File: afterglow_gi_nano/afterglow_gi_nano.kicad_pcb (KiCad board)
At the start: 2 copper layers, 52 parts, among them J1 Conn_02x17_Odd_Even, J2 POWER_CONN, J3 GI_WPC_J120, J4 GI_WPC_J121, J5 GI_CONN_J119, Q1 FQP30N06L, Q2 FQP30N06L, Q3 FQP30N06L, Q4 FQP30N06L, Q5 FQP30N06L, U1 74LS374, U2 L7805

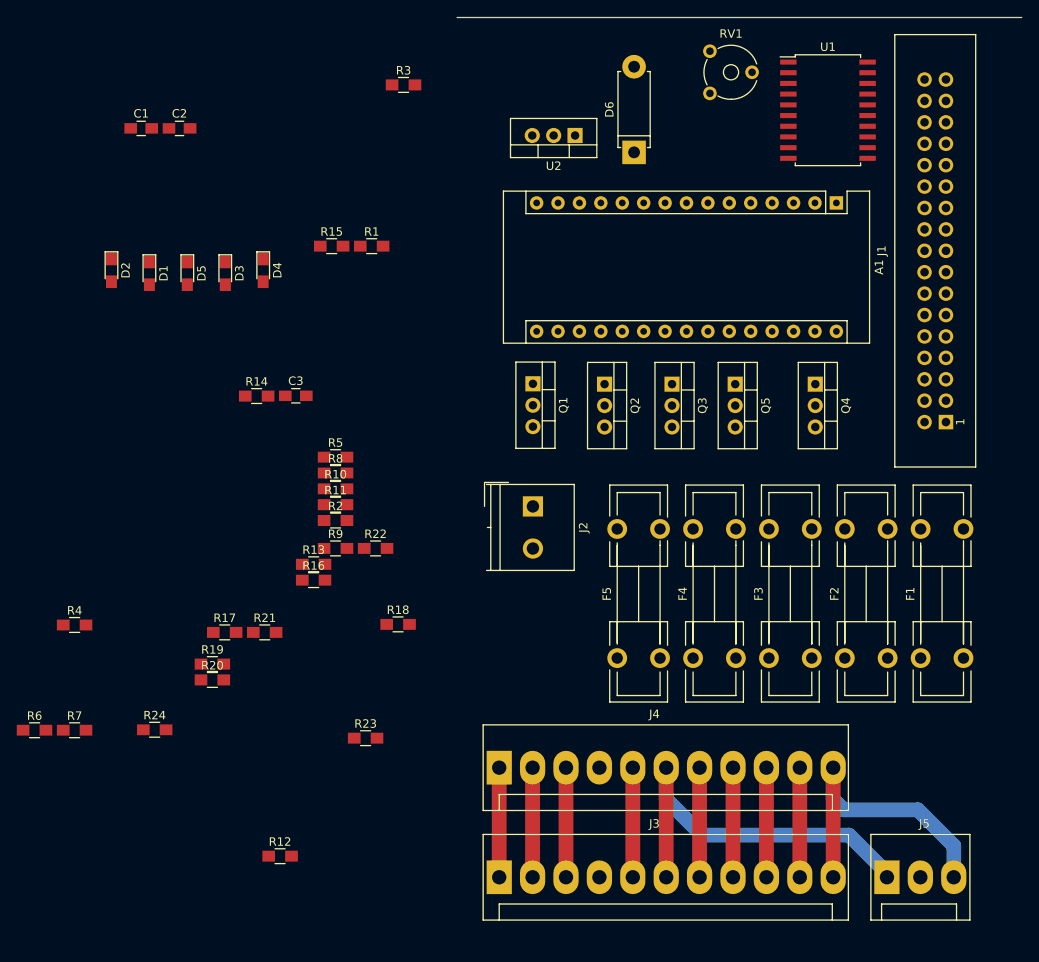
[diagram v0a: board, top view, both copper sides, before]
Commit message: Some PCB progress
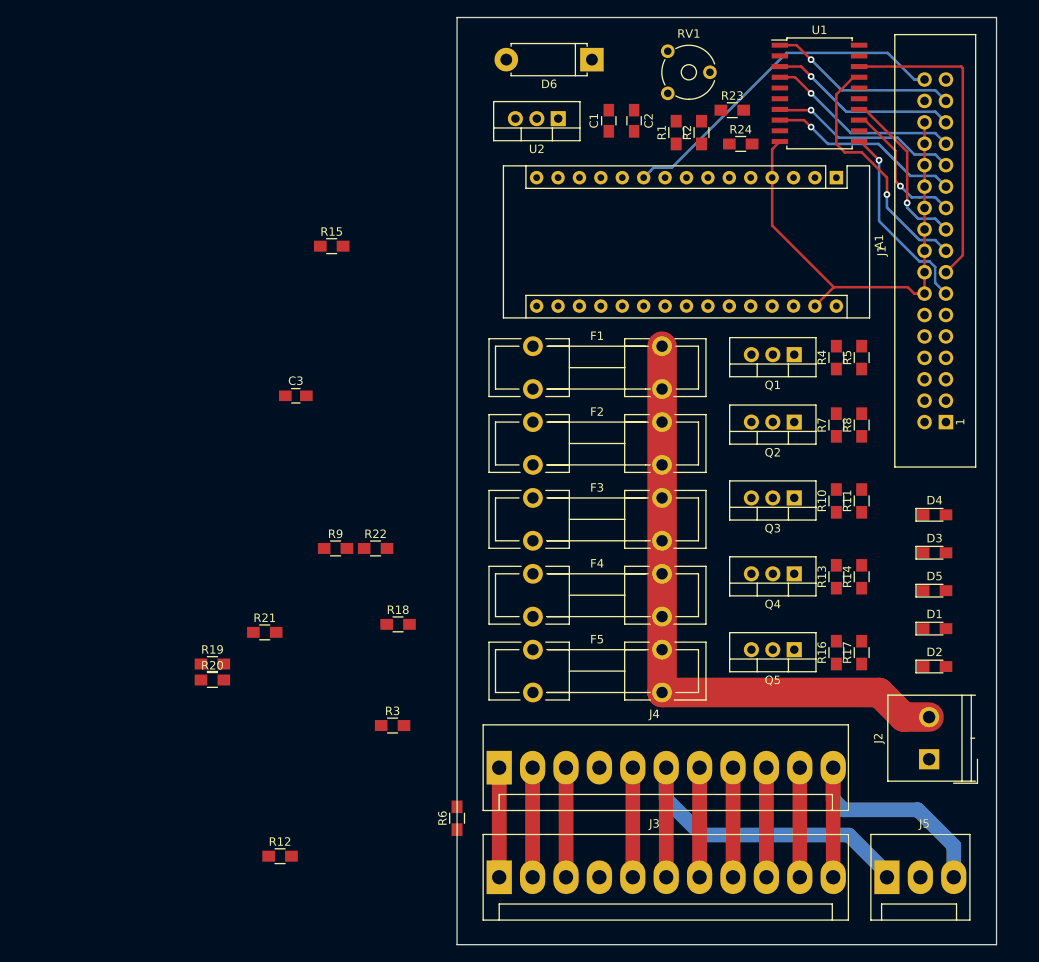
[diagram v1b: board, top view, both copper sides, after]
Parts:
- moved D2 108.4 mm to (110.7, 107.0), turned to 0 degrees
- moved D1 102.2 mm to (110.7, 102.5), turned to 0 degrees
- moved R24 98.3 mm to (87.7, 45.0)
- moved R7 97.4 mm to (99.0, 78.3), turned to 90 degrees
- moved D5 96.3 mm to (110.7, 98.0), turned to 0 degrees
- moved R4 95.8 mm to (99.0, 70.3), turned to 90 degrees
- moved D3 90.4 mm to (110.7, 93.5), turned to 0 degrees
- moved R23 86.3 mm to (86.7, 41.0)
- moved D4 84.8 mm to (110.7, 89.0), turned to 0 degrees
- moved R3 76.0 mm to (46.4, 114.0)
- moved R17 75.6 mm to (102.0, 105.3), turned to 90 degrees
- moved R14 74.9 mm to (102.0, 96.3), turned to 90 degrees
- moved R5 63.5 mm to (102.0, 70.3), turned to 90 degrees
- moved R2 63.3 mm to (83.0, 43.6), turned to 90 degrees
- moved R8 62.7 mm to (102.0, 78.3), turned to 90 degrees
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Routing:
- net +12V: track 0.00 -> 74.0 mm
- net GND: track 0.00 -> 55.3 mm
- net /ZC: track 0.00 -> 40.8 mm
- net /D7: track 0.00 -> 37.4 mm
- net /D6: track 0.00 -> 29.8 mm, vias 0 -> 1
- net /TRIAC: track 0.00 -> 23.1 mm, vias 0 -> 1
- net /D3: track 0.00 -> 23.0 mm, vias 0 -> 1
- net /D1: track 0.00 -> 23.0 mm, vias 0 -> 1
- net /BLANK: track 0.00 -> 22.4 mm, vias 0 -> 1
- net /D2: track 0.00 -> 22.4 mm, vias 0 -> 1
- net /D0: track 0.00 -> 22.4 mm, vias 0 -> 1
- net /D5: track 0.00 -> 20.1 mm, vias 0 -> 1
- net /D4: track 0.00 -> 16.7 mm, vias 0 -> 1
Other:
- board outline added: 64 x 110 mm
- net class Default: clearance 0.2 -> 0.25; trace_width 0.25 -> 0.3
- rule trace_clearance: 0.2 -> 0.25
